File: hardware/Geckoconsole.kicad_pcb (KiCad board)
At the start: 2 copper layers, 81.8 x 42.7 mm, 54 parts, among them J1 Conn_01x08_Male, J11 Conn_01x06_Male, J31 Conn_01x07_Female, J50 USB-C, J51 Conn_01x06_Male, J70 I²C, J81 Conn_01x07, Q51 S8050, Q52 S8050, SW2 Reset, SW41 Rotary_Encoder_Switch, U1 ESP32-WROOM-32, U101 AMS1117-3.3, U2 CP2102

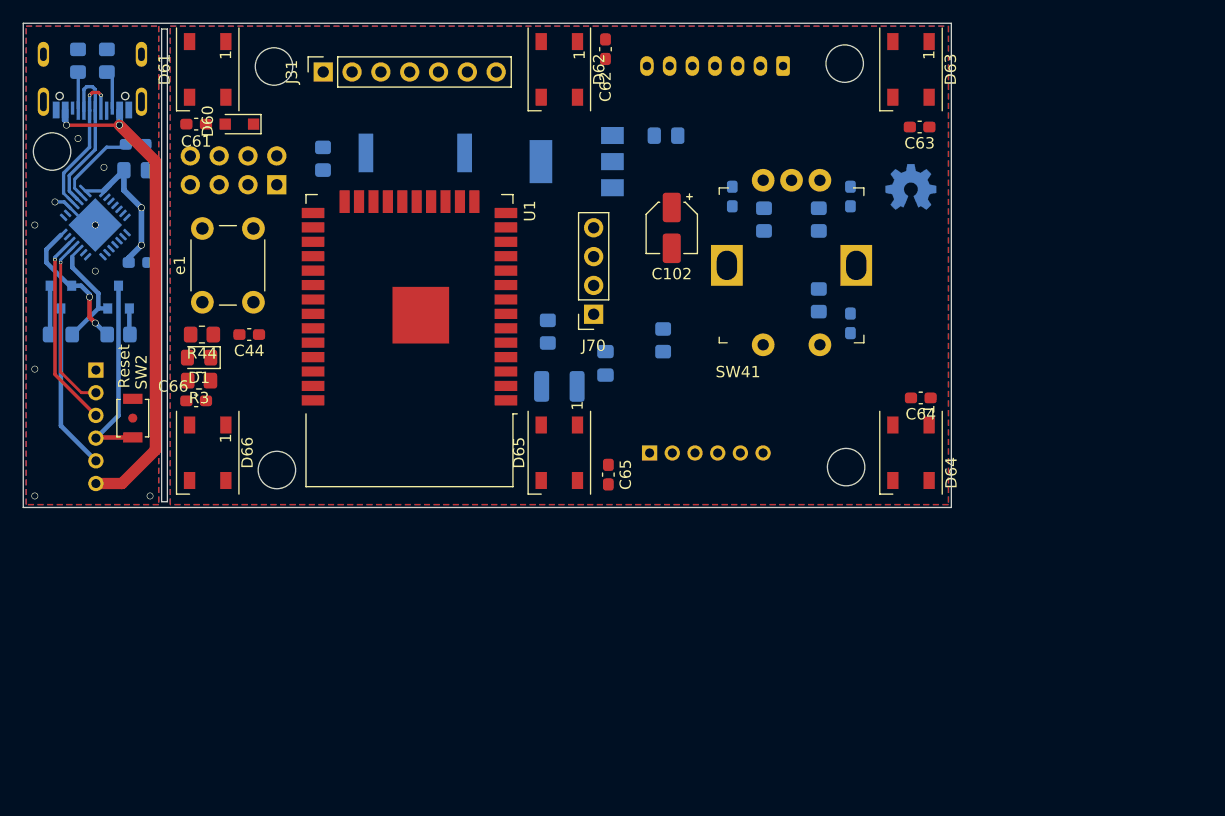
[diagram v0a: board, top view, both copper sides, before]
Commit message: Hardware Console: Route PCB, Pannelize
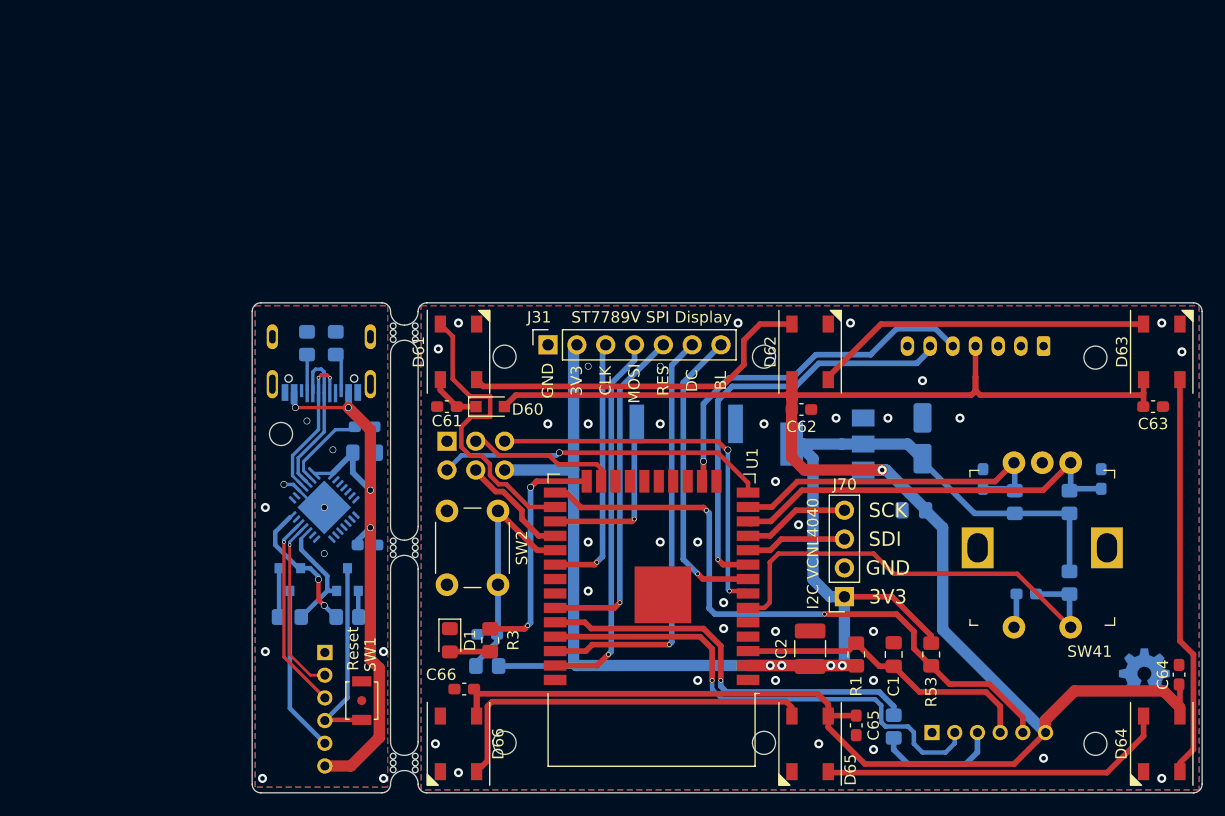
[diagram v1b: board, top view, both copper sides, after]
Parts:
- added G***: LOGO, Fraxinas:purplegecko, F.Cu at (93.0, 84.6)
- C1, C2, R1, R53: moved to F.Cu
- C102, C44, R44: moved to B.Cu
- D61, D62, D63, D64, D65, D66: footprint LED_SMD:LED_WS2812B_PLCC4_5.0x5.0mm_P3.2mm -> Fraxinas:LED_WS2812B_PLCC4_5.0x5.0mm_P3.2mm_Marking
- J1: value Conn_01x08_Male -> Conn_01x06_Male; footprint Connector_PinHeader_2.54mm:PinHeader_2x04_P2.54mm_Vertical -> Connector_PinHeader_2.54mm:PinHeader_2x03_P2.54mm_Vertical
- moved R53 69.1 mm to (117.9, 90.9)
- moved LOGO1 47.4 mm to (136.7, 93.5)
- moved R54 39.6 mm to (114.6, 97.3)
- moved C101 39.6 mm to (116.3, 78.2)
- moved R1 39.3 mm to (111.3, 90.9), turned to -90 degrees
- moved R44 38.5 mm to (78.7, 91.9), turned to 0 degrees
- moved C62 36.1 mm to (106.4, 69.3), turned to 0 degrees
- moved C1 36.1 mm to (114.6, 90.9), turned to 90 degrees
- moved J11 35.0 mm to (117.9, 97.8)
- moved C66 34.7 mm to (76.7, 94.0)
- moved R3 34.4 mm to (79.0, 89.7), turned to 90 degrees
- moved D66 33.9 mm to (76.2, 98.8)
- moved D65 33.9 mm to (107.2, 98.8)
- moved D64 33.9 mm to (138.2, 98.8)
- moved BZ1 33.8 mm to (96.3, 70.6)
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- renumbered SW2 to SW1, e1 to SW2
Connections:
- C61 pad 1: +5V -> Net-(C61-Pad1)
- D60 pad 1: Net-(D60-Pad1) -> Net-(C61-Pad1)
- D61 pad 1: Net-(D60-Pad1) -> Net-(C61-Pad1)
- J1 pad 2: GPIO02 -> GPIO12
- J1 pad 3: GPIO12 -> GPIO15
- J1 pad 4: GPIO15 -> GPIO17
- J1 pad 5: GPIO17 -> GPIO35
- J1 pad 6: GPIO35 -> +3V3
- R3 pad 2: GPIO02 -> Net-(R3-Pad2)
- U1 pad 12: ENC_B -> ENC_A
- U1 pad 13: ENC_A -> ENC_B
- U1 pad 24: GPIO02 -> Net-(R3-Pad2)
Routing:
- net +5V: track 60.2 -> 249.1 mm, vias 4 -> 5
- net +3V3: track 0.00 -> 139.7 mm, vias 0 -> 4
- net IO0: track 0.00 -> 56.5 mm, vias 0 -> 2
- net TXD0: track 0.00 -> 44.3 mm, vias 0 -> 1
- net ENC_SW: track 0.00 -> 41.3 mm
- net RX1: track 0.00 -> 37.7 mm, vias 0 -> 1
- net SPI_DC: track 0.00 -> 37.5 mm, vias 0 -> 1
- net ENC_A: track 0.00 -> 36.3 mm
- net RXD0: track 0.00 -> 35.8 mm, vias 0 -> 1
- net Net-(D63-Pad2): track 0.00 -> 34.8 mm
- net GPIO35: track 0.00 -> 34.2 mm, vias 0 -> 2
- net Net-(D65-Pad2): track 0.00 -> 33.4 mm
- net SPI_MOSI: track 0.00 -> 33.3 mm, vias 0 -> 1
- net TX1: track 0.00 -> 32.2 mm, vias 0 -> 1
- net Net-(D61-Pad2): track 0.00 -> 31.6 mm
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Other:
- board size 81.8 x 42.7 mm -> 83.7 x 43.2 mm
- board text added: "12 17 3V3"
- board text added: "3V3"
- board text added: "5V"
- board text added: "BL"
- board text added: "CLK"
- board text added: "DC"
- board text added: "GND"
- board text added: "GND 15 35"
- board text added: "I2C VCNL4040"
- board text added: "MH-Z19 CO2 Sensor"
- board text added: "MOSI"
- board text added: "RES"
- board text added: "SCK"
- board text added: "SDI"
- board text added: "ST7789V SPI Display"
- board text added: "►"
- board text added: "◄"
- board text removed: "Reset"
